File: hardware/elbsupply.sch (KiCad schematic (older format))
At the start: 76 parts

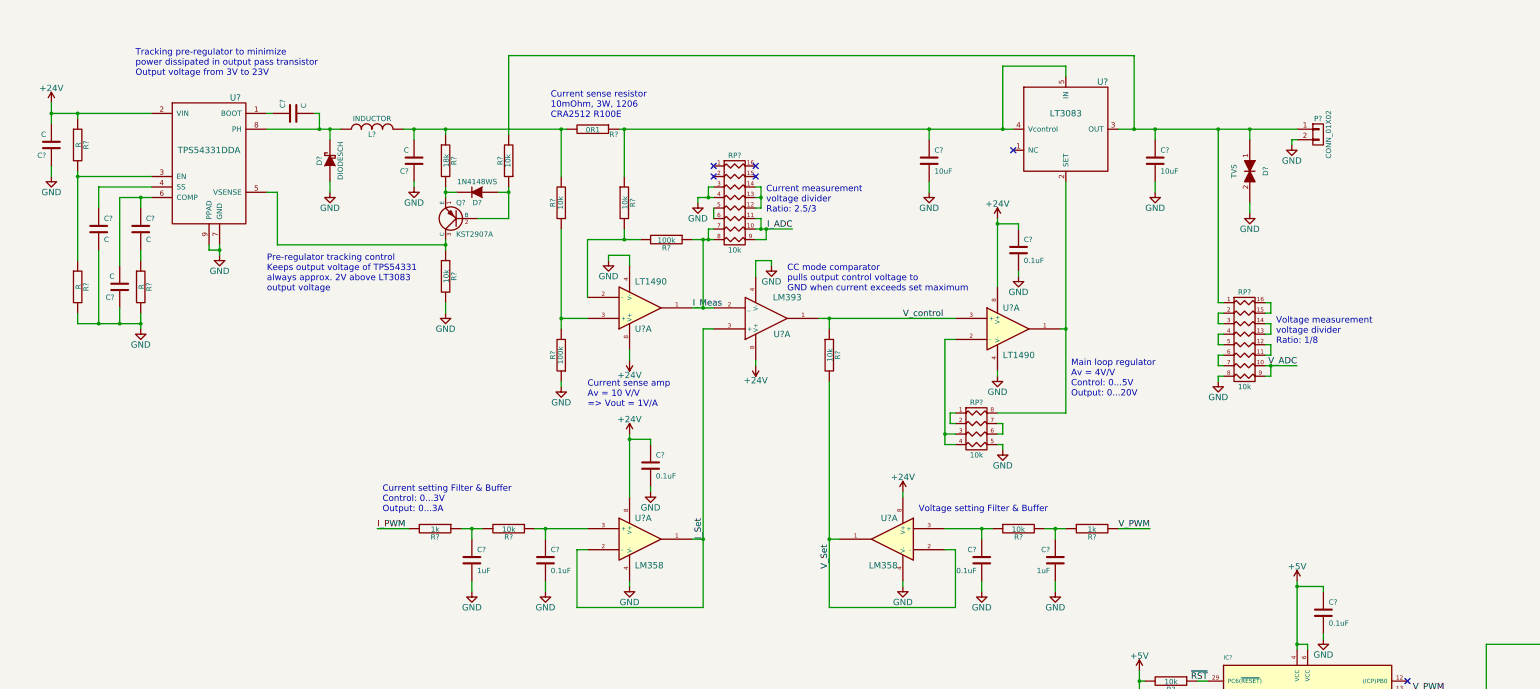
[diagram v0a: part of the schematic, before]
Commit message: final Rev. A schematic
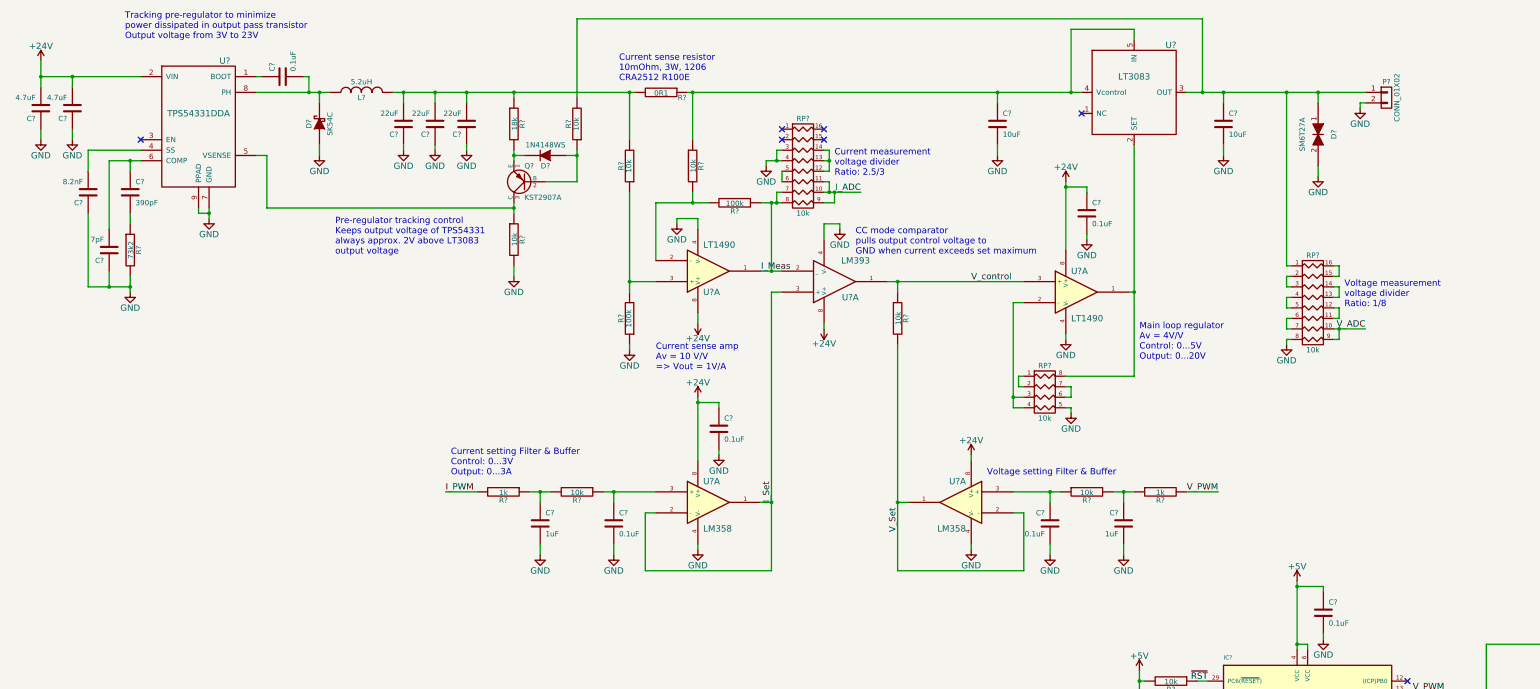
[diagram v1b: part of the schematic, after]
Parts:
- removed R? (x2): R, symbol R
- added C?: 4.7uF, symbol C
- added C? (x2): 22uF, symbol C
- C?: value C -> 0.1uF
- C?: value C -> 22uF
- C?: value C -> 390pF
- C?: value C -> 7pF
- C?: value C -> 8.2nF
- C?: value C -> 4.7uF
- D?: value DIODESCH -> SK54C
- D?: value TVS -> SM6T27A
- L?: value INDUCTOR -> 5.2uH
- R?: value R -> 73k2
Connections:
- net +24V: now also C?.2
- net GND: now also C?.1, C?.1, C?.1, C?.1; no longer C?.2
- net at C?.2, L?.2, R?.1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: now also C?.2, C?.2
- net at U?.4 (SS): now also C?.2; no longer C?.1
- no-connect marks 15 -> 16
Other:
- moved on the sheet: C?, D?, L?, P?, Q?, R?, RP?, U?, U?A
